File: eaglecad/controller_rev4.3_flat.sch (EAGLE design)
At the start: 110 parts, among them U100 STM32L452XX_QFPN48, U101 TCAN330, U200 TPS63070, U300 STSPIN230, U301 TSV991ILT, U302 AS5047P, U400 STSPIN250, U401 TSV991ILT, X101 ABM10-16MHz

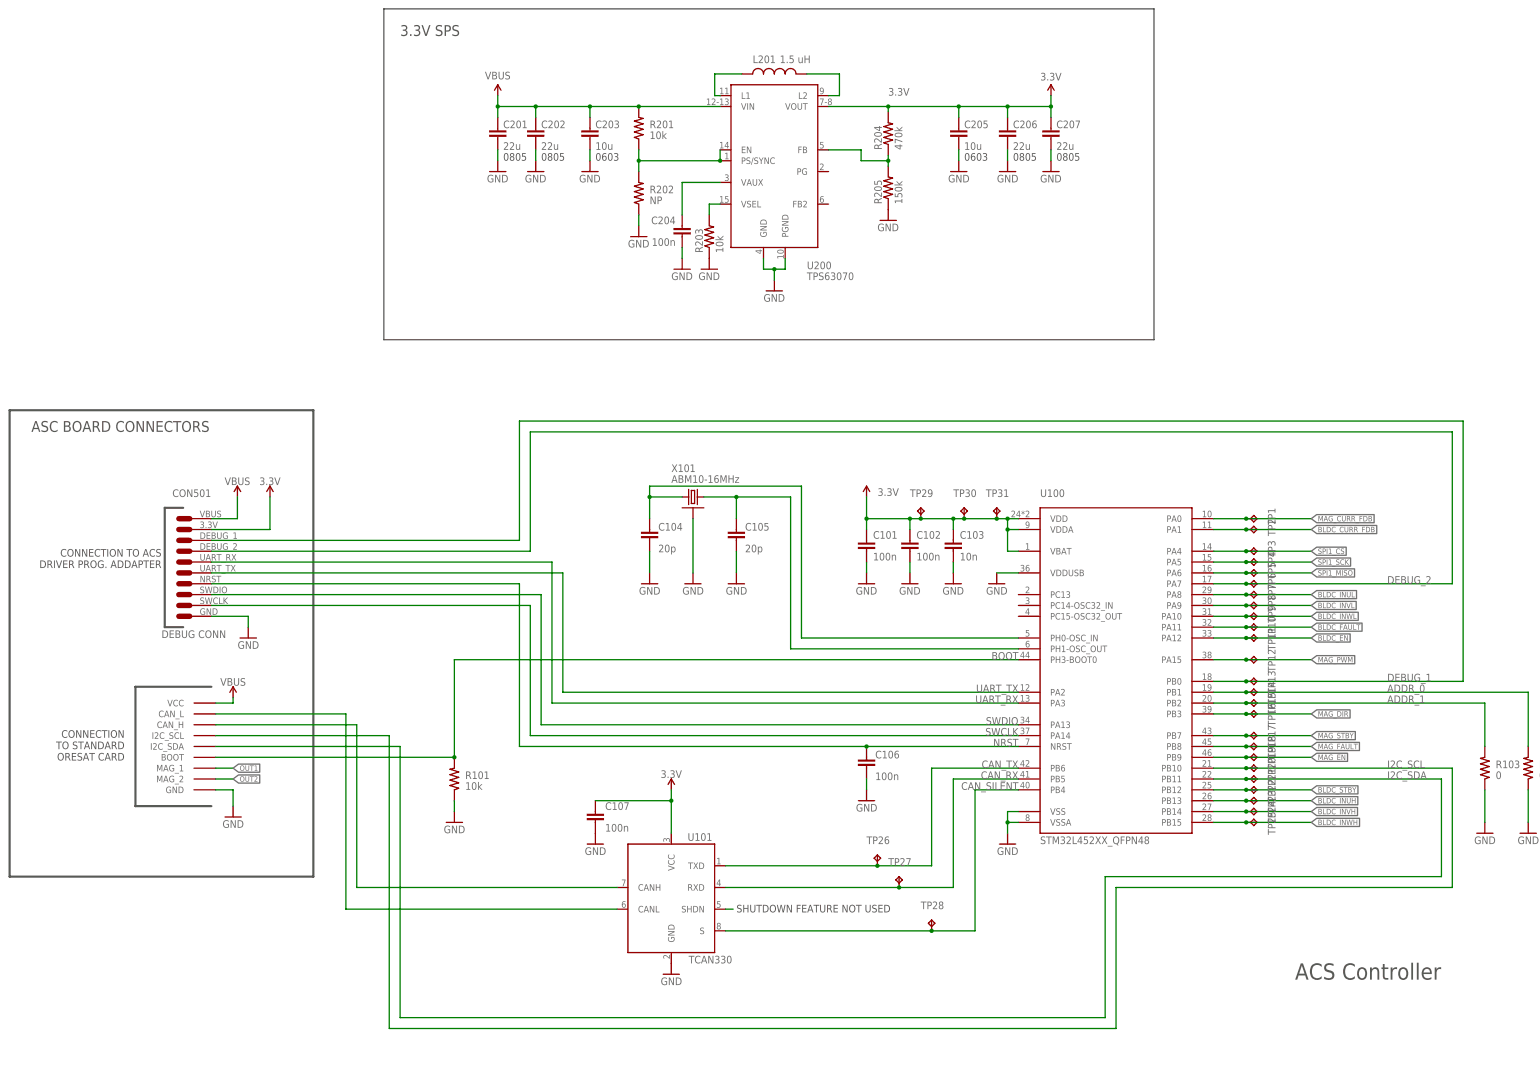
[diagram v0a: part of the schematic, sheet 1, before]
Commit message: Flattening the board
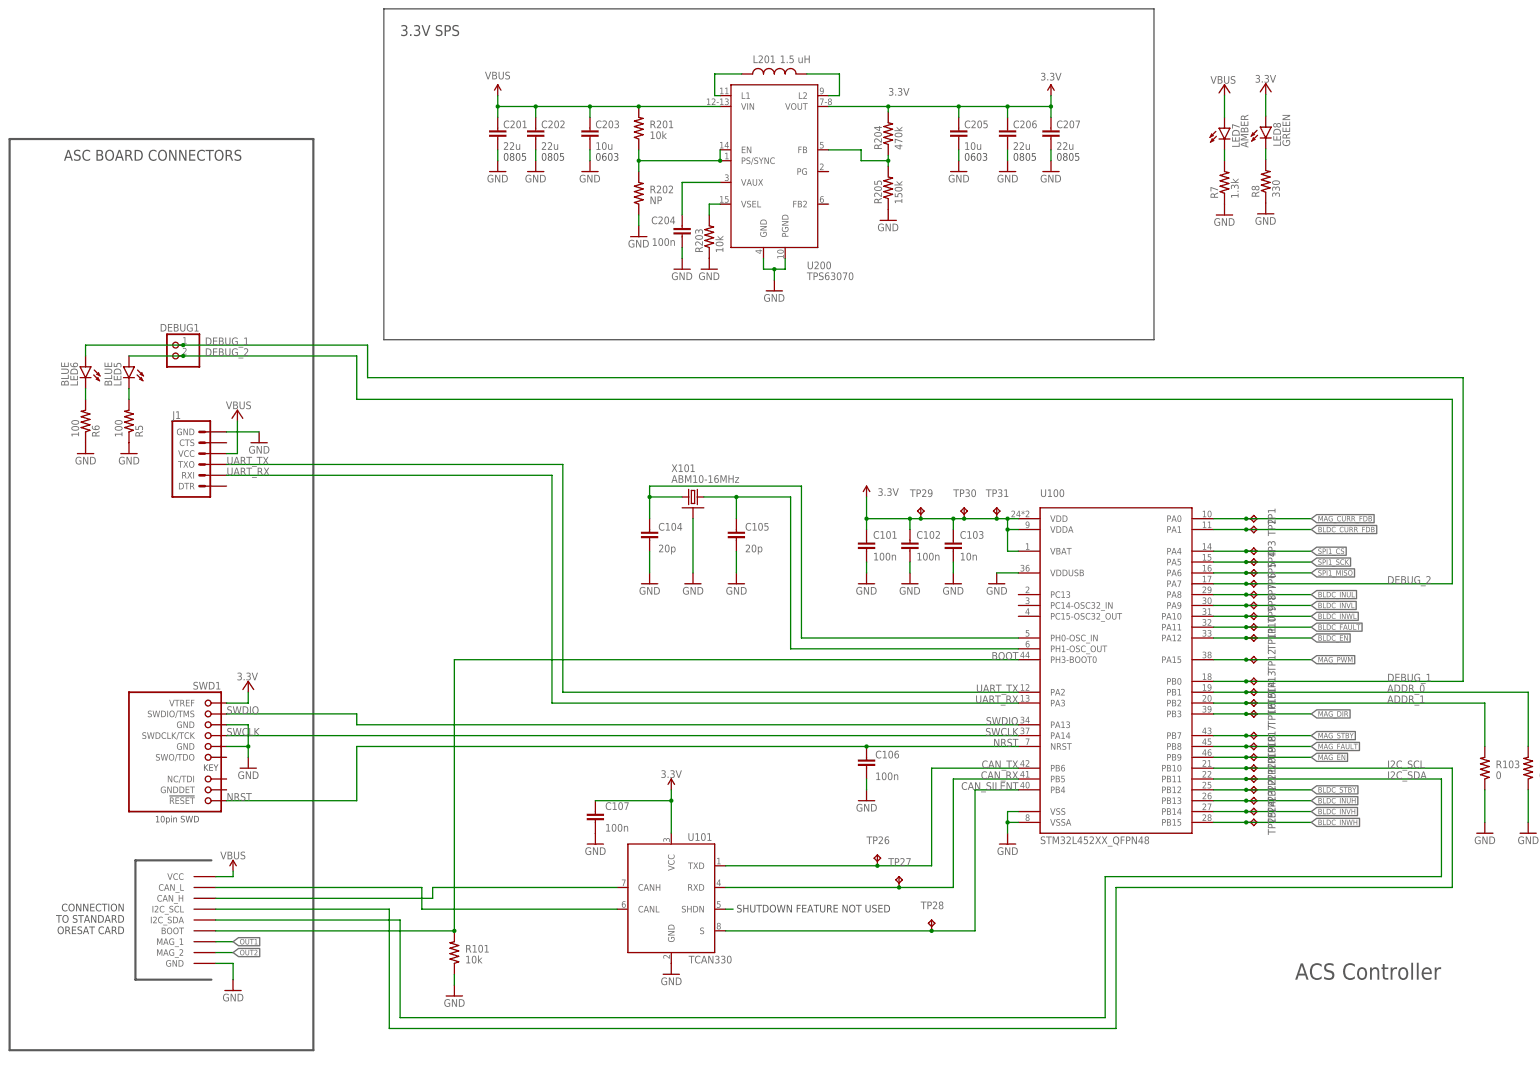
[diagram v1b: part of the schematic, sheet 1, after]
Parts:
- removed C501: DEBUG_CON, oresat-ACS_driver_board:DEBUG_CON
- added DEBUG1: (no value), pinhead:PINHD-1X2
- added J1: (no value), SparkFun-Connectors:6_PIN_SERIAL_TARGETSILK
- added LED5, LED6: BLUE, led:LEDCHIPLED_0603
- added LED7: AMBER, led:LEDCHIPLED_0603
- added LED8: GREEN, led:LEDCHIPLED_0603
- added R5, R6: 100, oresat-rcl:R-US_0402-B-NOSILK
- added R7: 1.3k, oresat-rcl:R-US_0402-B-NOSILK
- added R8: 330, oresat-rcl:R-US_0402-B-NOSILK
- added SWD1: 1.27MM-SWD-CONNECTOR, J-CNC-3220-10-0100-00-ARM-SWD-port:1.27MM-SWD-CONNECTOR
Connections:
- new net N$5: LED5.C, R5.2
- new net N$6: LED6.C, R6.2
- new net N$7: LED7.C, R7.2
- new net N$8: LED8.C, R8.2
- net 3.3V: now also LED8.A, SWD1.VTREF; no longer C501.2
- net DEBUG_1: now also DEBUG1.1, LED6.A; no longer C501.3
- net DEBUG_2: now also DEBUG1.2, LED5.A; no longer C501.4
- net GND: now also J1.GND, R5.1, R6.1, R7.1, R8.1, SWD1.GND, SWD1.GND@2; no longer C501.10
- net NRST: now also SWD1.!RESET; no longer C501.7
- net SWCLK: now also SWD1.SWDCLK/TCK; no longer C501.9
- net SWDIO: now also SWD1.SWDIO/TMS; no longer C501.8
- net UART_RX: now also J1.RXI; no longer C501.5
- net UART_TX: now also J1.TXO; no longer C501.6
- net VBUS: now also J1.VCC, LED7.A; no longer C501.1
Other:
- note removed: "CON501"
- note removed: "CONNECTION TO ACS DRIVER PROG. ADDAPTER"
- note removed: "DEBUG CONN"
- moved on the sheet: R101
